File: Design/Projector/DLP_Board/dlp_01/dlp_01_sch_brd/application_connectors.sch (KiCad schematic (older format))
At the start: 15 parts

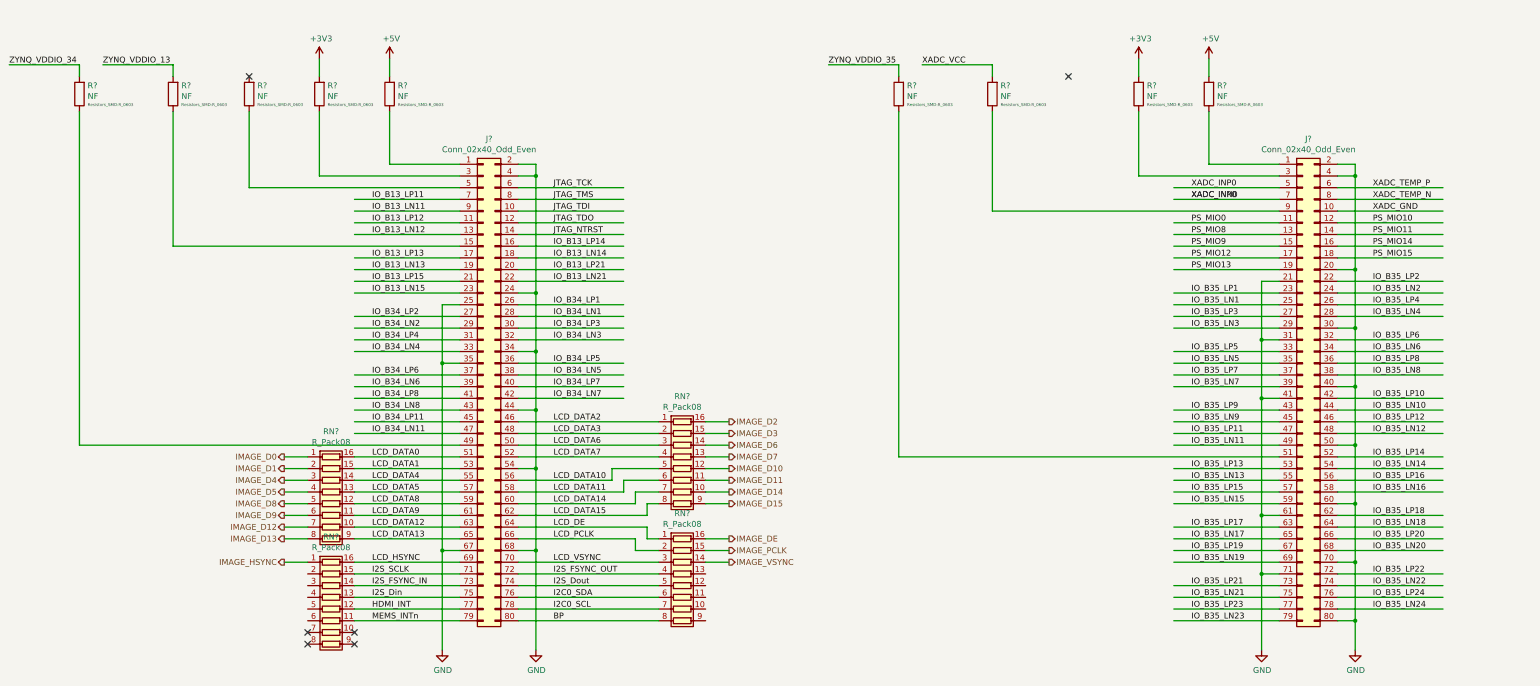
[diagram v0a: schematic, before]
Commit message: Ongoing updates the schematics
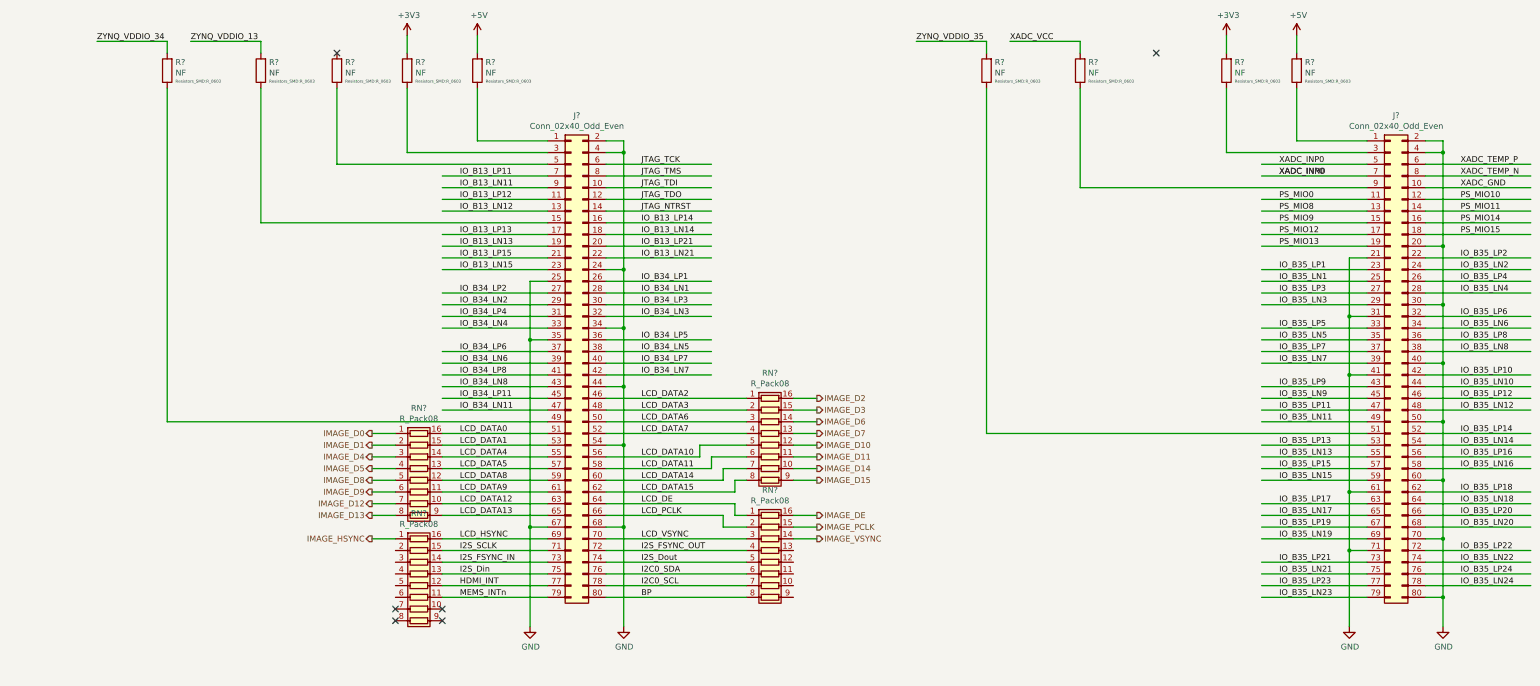
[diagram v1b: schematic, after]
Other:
- moved on the sheet: J?, R?, RN?
